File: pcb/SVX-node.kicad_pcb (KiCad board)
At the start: 4 copper layers, 48.2 x 46.2 mm, 0 parts

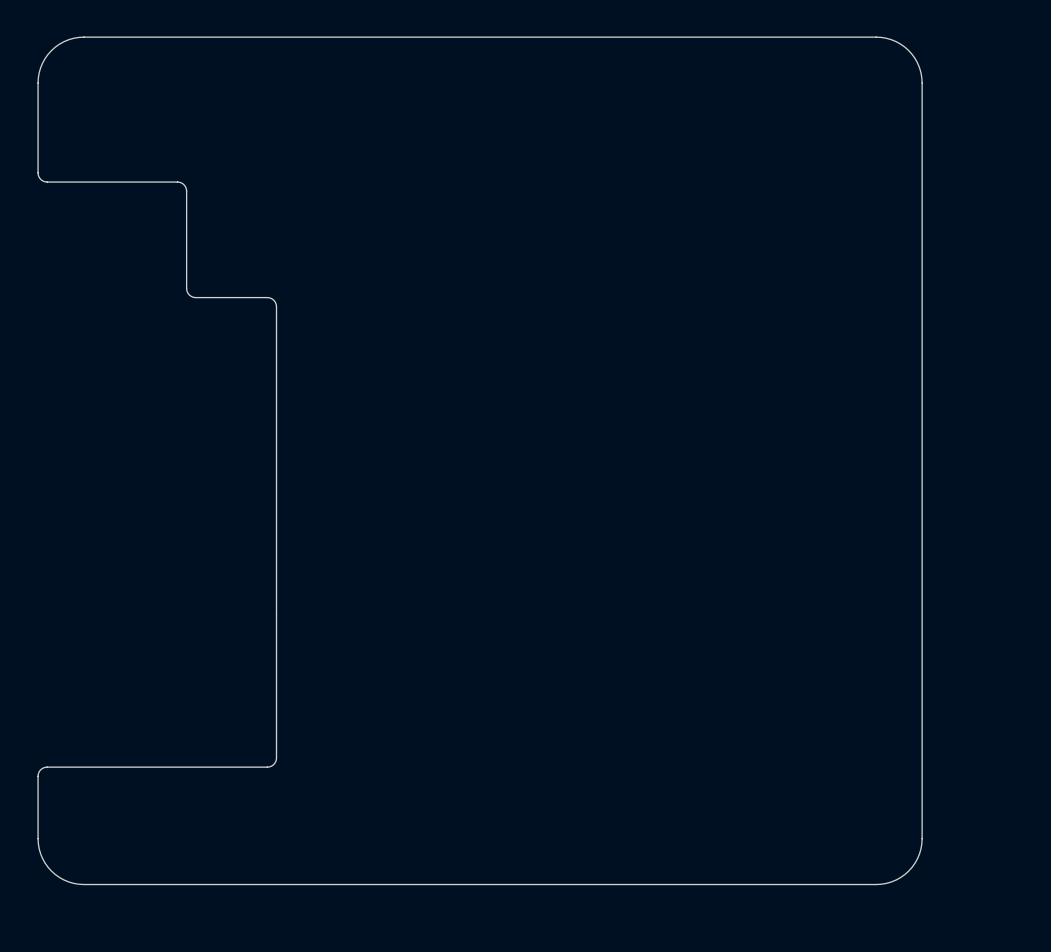
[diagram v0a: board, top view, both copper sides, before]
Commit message: feat: Finalize pcb layout for protoboard assembly
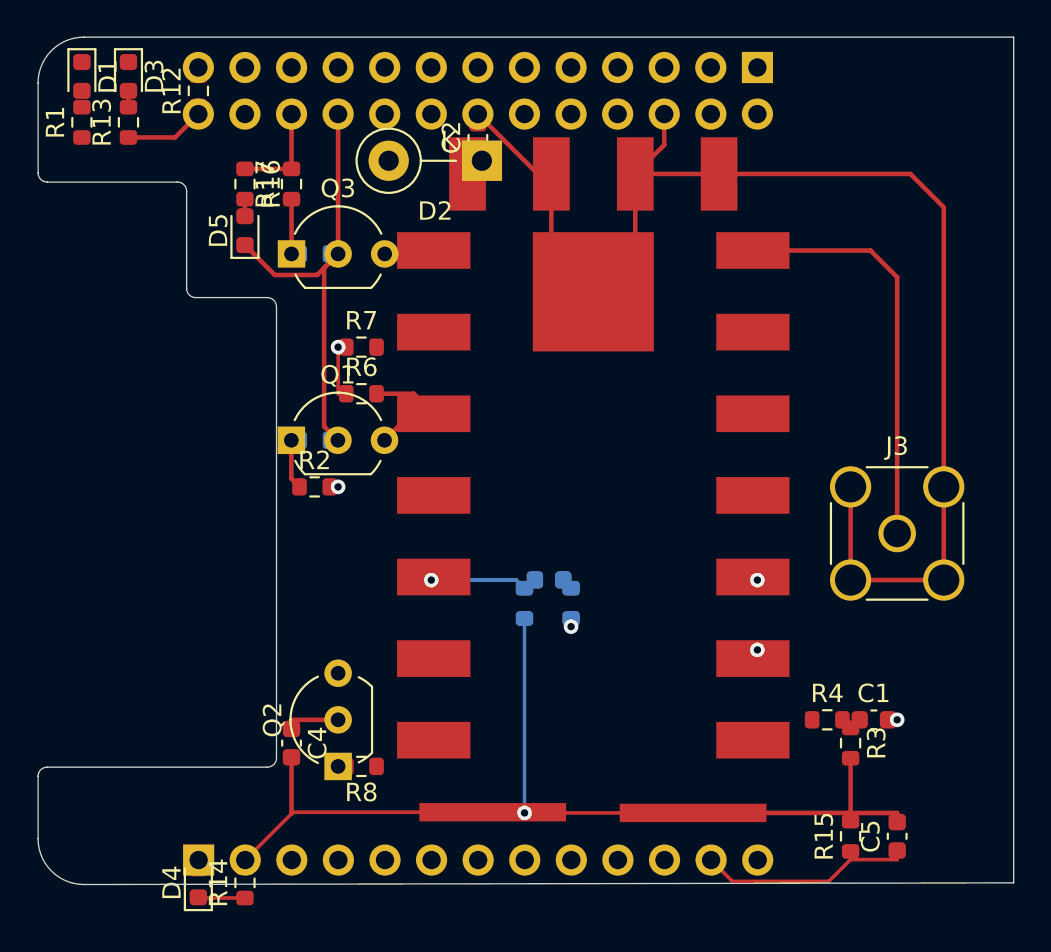
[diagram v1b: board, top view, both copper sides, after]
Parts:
- added C1: 470nF, Capacitor_SMD:C_0603_1608Metric, F.Cu at (204.5, 71.1)
- added C2: 0,1uF, Capacitor_SMD:C_0603_1608Metric, F.Cu at (182.9, 39.4)
- added C3: 470nF, Capacitor_SMD:C_0603_1608Metric, B.Cu at (186.8, 63.5)
- added C4: 0,1uF, Capacitor_SMD:C_0603_1608Metric, F.Cu at (172.7, 72.4)
- added C5: 470nF, Capacitor_SMD:C_0603_1608Metric, F.Cu at (205.7, 77.5)
- added D1: PTT, LED_SMD:LED_0603_1608Metric, F.Cu at (161.3, 36.0)
- added D2: 1N4001, Diode_THT:D_DO-41_SOD81_P5.08mm_Vertical_KathodeUp, F.Cu at (183.1, 40.6)
- added D3: SQL, LED_SMD:LED_0603_1608Metric, F.Cu at (163.8, 36.0)
- added D4: 5V, LED_SMD:LED_0603_1608Metric, F.Cu at (167.6, 80.0)
- added D5: Low-power, LED_SMD:LED_0603_1608Metric, F.Cu at (170.2, 44.5)
- added J1: Conn_02x13_Odd_Even, Connector_PinSocket_2.54mm:PinSocket_2x13_P2.54mm_Vertical, B.Cu at (198.1, 35.6)
- added J2: Conn_01x13, Connector_PinSocket_2.54mm:PinSocket_1x13_P2.54mm_Vertical, B.Cu at (167.7, 78.8)
- added J3: Conn_Coaxial, Connector_Coaxial:SMA_Amphenol_132291-12_Vertical, F.Cu at (205.7, 61.0)
- added Q1: Q_NPN_BEC, Package_TO_SOT_THT:TO-92_Inline_Wide, F.Cu at (172.7, 55.9)
- added Q2: Q_PNP_BEC, Package_TO_SOT_THT:TO-92_Inline_Wide, F.Cu at (175.3, 73.7)
- added Q3: Q_NPN_BEC, Package_TO_SOT_THT:TO-92_Inline_Wide, F.Cu at (172.7, 45.7)
- added R1: 330R, Resistor_SMD:R_0603_1608Metric, F.Cu at (161.3, 38.5)
- added R10: 2K2, Resistor_SMD:R_0603_1608Metric, B.Cu at (188.0, 64.8)
- added R11: 1K, Resistor_SMD:R_0603_1608Metric, B.Cu at (185.4, 64.8)
- added R12: 10K, Resistor_SMD:R_0603_1608Metric, F.Cu at (167.6, 36.8)
- added R13: 330R, Resistor_SMD:R_0603_1608Metric, F.Cu at (163.8, 38.5)
- added R14: 470R, Resistor_SMD:R_0603_1608Metric, F.Cu at (170.2, 80.0)
- added R15: 2K2, Resistor_SMD:R_0603_1608Metric, F.Cu at (203.2, 77.5)
- added R16: 330R, Resistor_SMD:R_0603_1608Metric, F.Cu at (170.2, 41.9)
- added R17: 2K2, Resistor_SMD:R_0603_1608Metric, F.Cu at (172.7, 41.9)
- added R18: 47K, Resistor_SMD:R_0603_1608Metric, B.Cu at (174.0, 45.7)
- added R2: 2K2, Resistor_SMD:R_0603_1608Metric, F.Cu at (174.0, 58.4)
- added R3: 1K, Resistor_SMD:R_0603_1608Metric, F.Cu at (203.2, 72.4)
- added R4: 10K, Resistor_SMD:R_0603_1608Metric, F.Cu at (201.9, 71.1)
- added R5: 47K, Resistor_SMD:R_0603_1608Metric, B.Cu at (174.0, 55.9)
- added R6: 4K7, Resistor_SMD:R_0603_1608Metric, F.Cu at (176.5, 53.3)
- added R7: 10K, Resistor_SMD:R_0603_1608Metric, F.Cu at (176.5, 50.8)
- added R8: 2K2, Resistor_SMD:R_0603_1608Metric, F.Cu at (176.5, 73.7)
- added R9: 47K, Resistor_THT:R_Axial_DIN0204_L3.6mm_D1.6mm_P5.08mm_Horizontal, B.Cu at (175.3, 73.7)
- added U1: SA868, SA868:SA868, F.Cu at (189.2, 58.9)
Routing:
- net GND: track 0.00 -> 151.0 mm, vias 0 -> 1
- net GPIO_10: track 0.00 -> 40.6 mm, vias 0 -> 1
- net +5V: track 0.00 -> 37.5 mm, vias 0 -> 2
- net UART_RX: track 0.00 -> 33.4 mm, vias 0 -> 1
- net UART_TX: track 0.00 -> 28.6 mm, vias 0 -> 1
- net LINEOUT_R: track 0.00 -> 27.5 mm, vias 0 -> 1
- net GPIO_13: track 0.00 -> 25.6 mm, vias 0 -> 2
- net /RF_OUT: track 0.00 -> 22.4 mm
- net MIC1P: track 0.00 -> 15.6 mm, vias 0 -> 1
- net MIC1N: track 0.00 -> 12.1 mm
- net Net-(Q1-Pad3): track 0.00 -> 6.41 mm
- net GPIO_2: track 0.00 -> 5.53 mm
- net Net-(C3-Pad2): track 0.00 -> 5.26 mm, vias 0 -> 1
- net +3V3: track 0.00 -> 3.03 mm
- net Net-(Q3-Pad1): track 0.00 -> 2.98 mm
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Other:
- board size 48.2 x 46.2 mm -> 53.2 x 46.2 mm
- board text removed: "46.0"
- board text removed: "48.0"
- board text removed: "GND"
- board text removed: "RX"
- board text removed: "TX"
